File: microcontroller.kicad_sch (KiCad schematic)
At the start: 1 part, among them U1 ESP32-WROOM-32E

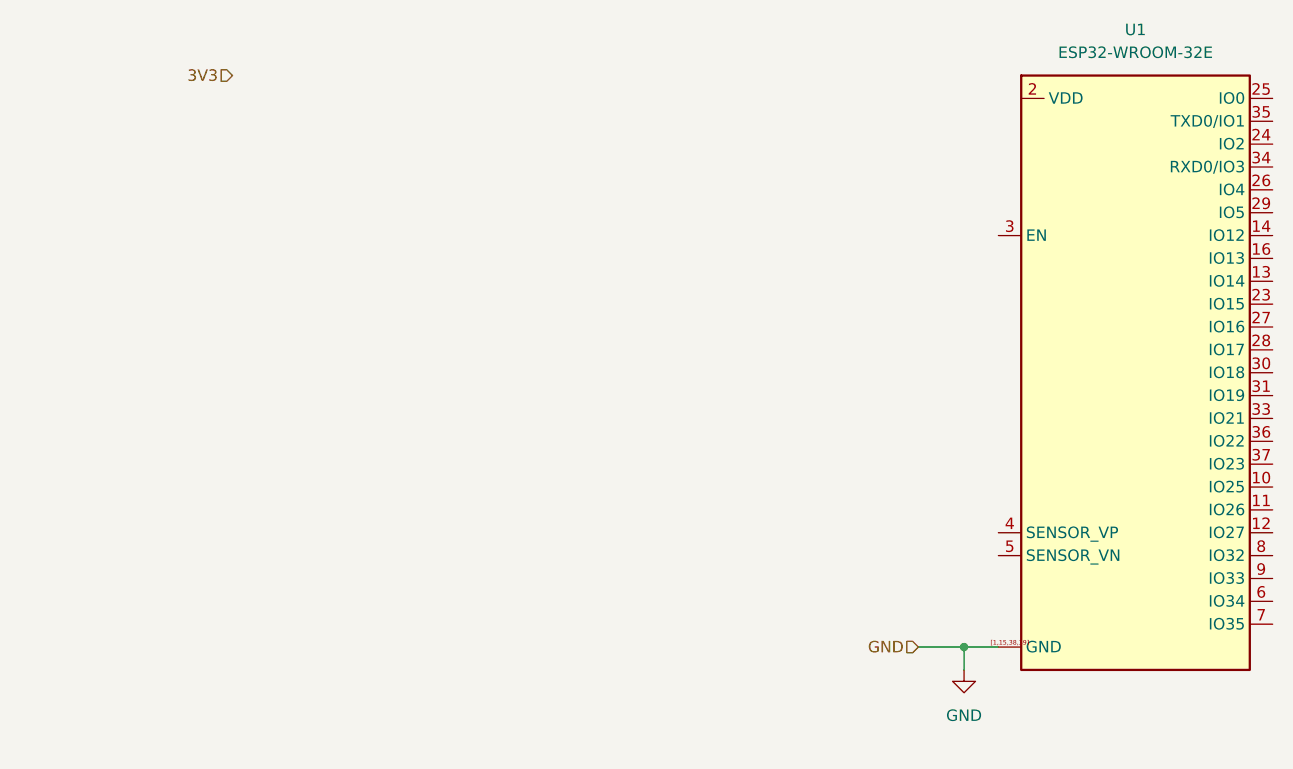
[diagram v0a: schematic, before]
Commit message: Adding ethernet module and more
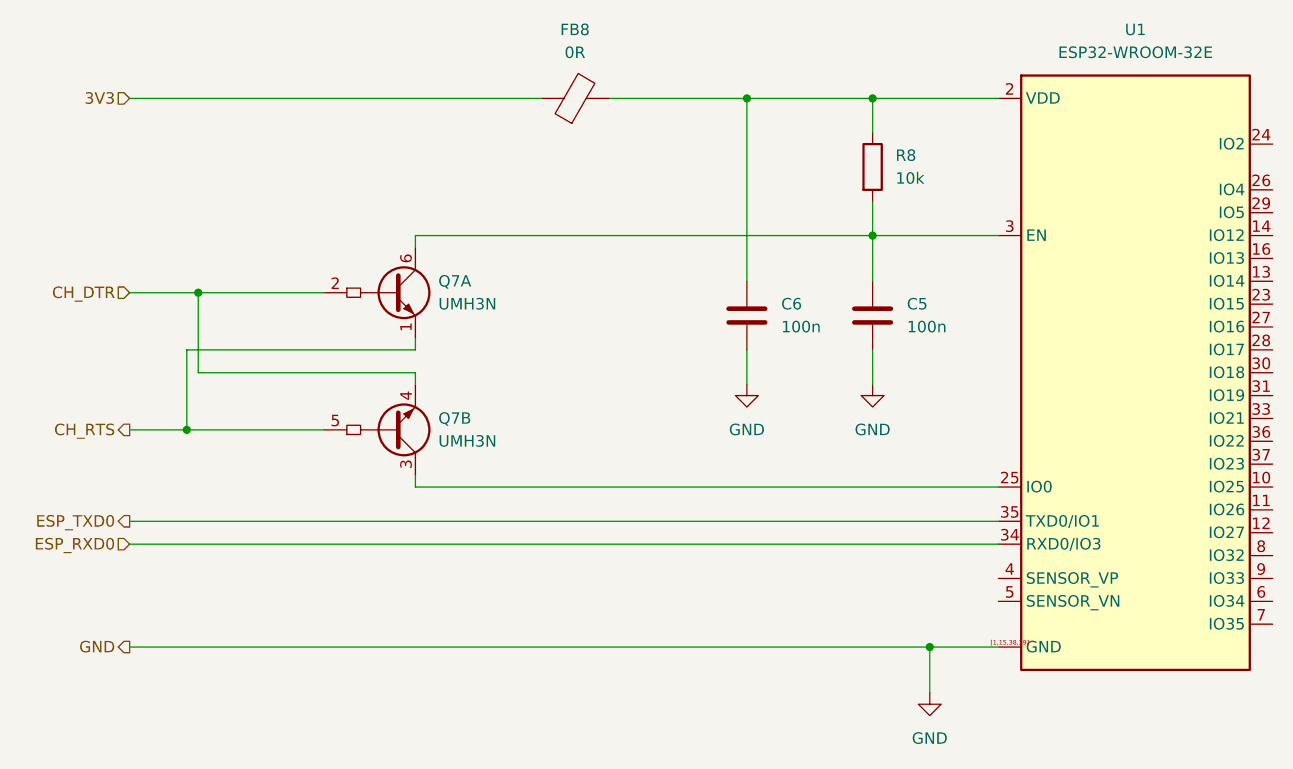
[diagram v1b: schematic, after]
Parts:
- added C5, C6: 100n, symbol Device:C
- added FB8: 0R, Inductor_SMD:L_0603_1608Metric, symbol Device:FerriteBead
- added Q7: UMH3N, Package_TO_SOT_SMD:SOT-363_SC-70-6, symbol Transistor_BJT:UMH3N
- added R8: 10k, symbol Device:R
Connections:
- net 3V3: now also FB8.1
- net GND: now also C5.2, C6.2
- net at U1.2 (VDD): now also C6.1, FB8.2, R8.1
- net at U1.25 (IO0): now also Q7.3 (C2)
- net at U1.3 (EN): now also C5.1, Q7.6 (C1), R8.2
- net ESP_RXD0: now reaches U1.34 (RXD0/IO3)
- net ESP_TXD0: now reaches U1.35 (TXD0/IO1)
- new net CH_DTR: Q7.2 (B1), Q7.4 (E2)
- new net CH_RTS: Q7.1 (E1), Q7.5 (B2)
